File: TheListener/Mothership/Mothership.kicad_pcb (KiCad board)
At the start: 2 copper layers, 81 parts, among them J1 RJ45, J2 RJ45, J3 RJ45, J4 RJ45, J5 RJ45, J6 RJ45, J7 RJ45, J8 RJ45, J9 Conn_01x02_Female, U1 SP3491, U10 AMS1117-3.3, U11 NID35-5, U12 Teensy3.5, U2 SP3491, U3 SP3491, U4 SP3491, U5 SP3491, U6 SP3491, U7 SP3491, U8 SP3491, U9 AMS1117-3.3

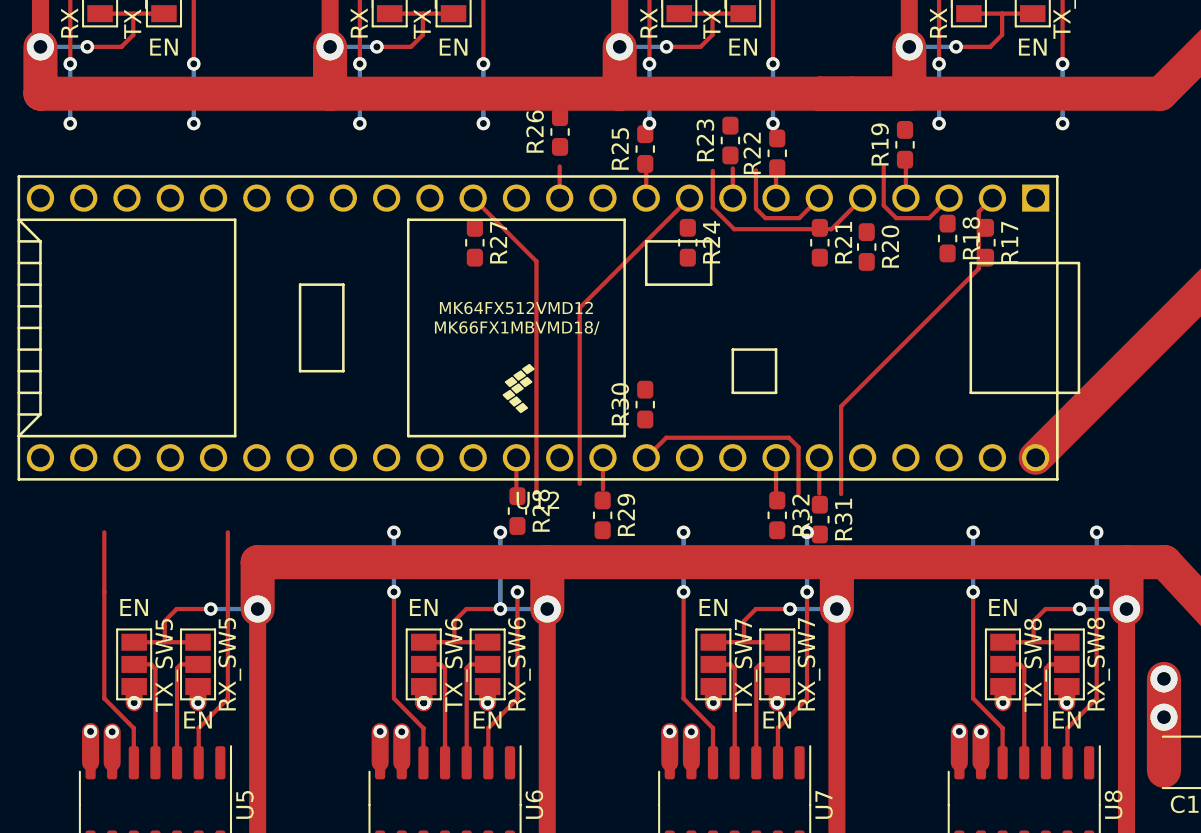
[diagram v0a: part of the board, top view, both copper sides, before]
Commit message: wip
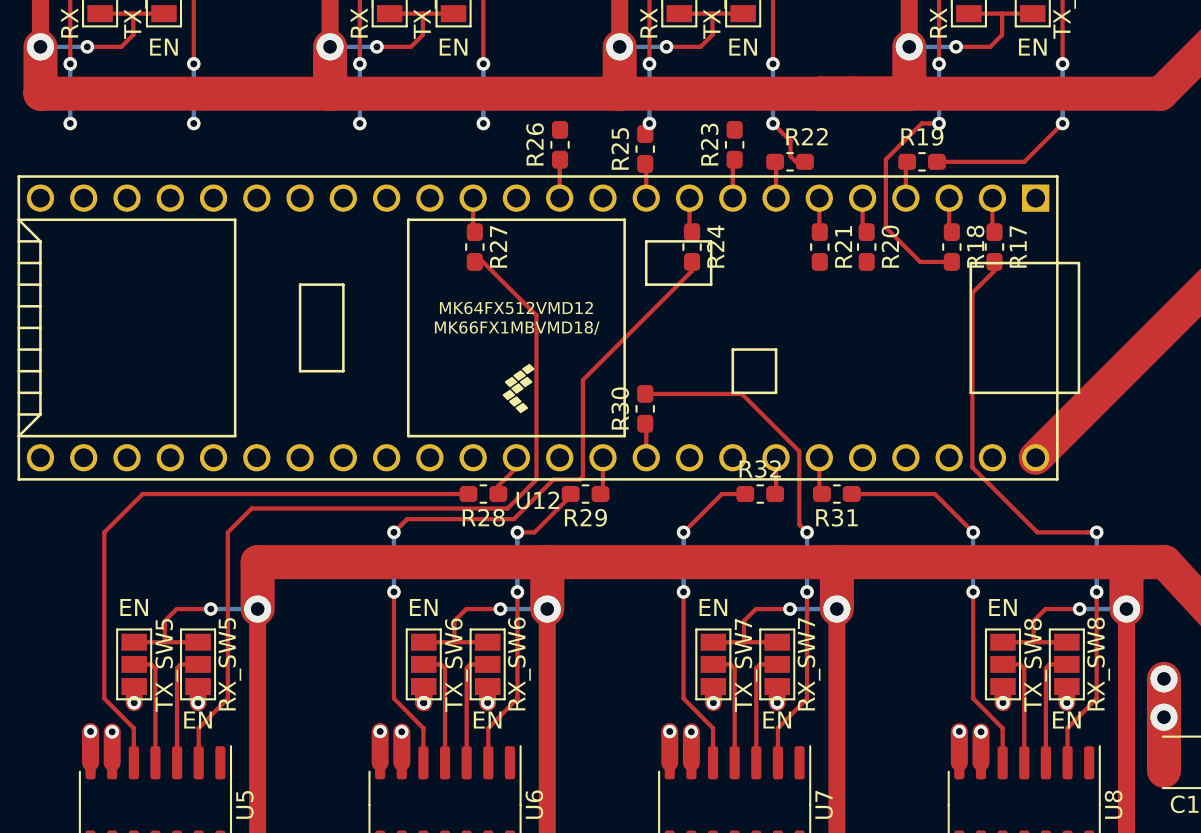
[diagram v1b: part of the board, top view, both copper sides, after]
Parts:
- moved R28 2.24 mm to (73.5, 89.0), turned to 180 degrees
- moved R31 1.80 mm to (94.2, 89.0), turned to 180 degrees
- moved R29 1.60 mm to (79.5, 89.0), turned to 180 degrees
- moved R32 1.60 mm to (89.8, 89.0), turned to 0 degrees
- moved R19 1.41 mm to (99.2, 69.5), turned to 0 degrees
- moved R22 0.90 mm to (91.5, 69.5), turned to 0 degrees
- moved R26 0.75 mm to (78.0, 68.5)
- moved R17 0.56 mm to (103.5, 74.5)
- moved R18 0.56 mm to (101.0, 74.5)
- moved R23 0.35 mm to (88.2, 68.5)
- moved R24 0.35 mm to (85.8, 74.5)
- moved R21 0.25 mm to (93.2, 74.5)
- moved R27 0.25 mm to (73.0, 74.5)
- moved R30 0.25 mm to (83.0, 84.0)
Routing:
- net R_5: track 14.3 -> 48.2 mm
- net T_6: track 14.3 -> 42.0 mm
- net T_5: track 14.3 -> 36.6 mm
- net R_8: track 14.3 -> 35.7 mm
- net Net-(R17-Pad1): track 21.0 -> 2.00 mm
- net Net-(R24-Pad1): track 19.4 -> 1.97 mm
- net Net-(R27-Pad1): track 18.8 -> 2.02 mm
- net R_7: track 14.3 -> 29.6 mm
- net R_1: track 14.3 -> 27.0 mm
- net Net-(R30-Pad1): track 12.4 -> 1.81 mm
- net Net-(R20-Pad1): track 12.2 -> 1.88 mm
- net T_1: track 14.3 -> 22.6 mm
- net T_8: track 14.3 -> 22.3 mm
- net R_6: track 10.8 -> 18.4 mm, vias 1 -> 2
- net Net-(R18-Pad1): track 6.95 -> 1.71 mm
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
